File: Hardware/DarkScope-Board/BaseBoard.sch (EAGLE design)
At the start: 87 parts, among them IC1 7805DT, IC2 REG1117, IC3 7905, J1 DCJ0202, Q1 8MHz, T2 9014, U1 STM32F103CBT6, X1 TSW-102-07-G-S, X2 TSW-102-07-G-S, X3 MINI-USB-32005-301, X4 2540-5

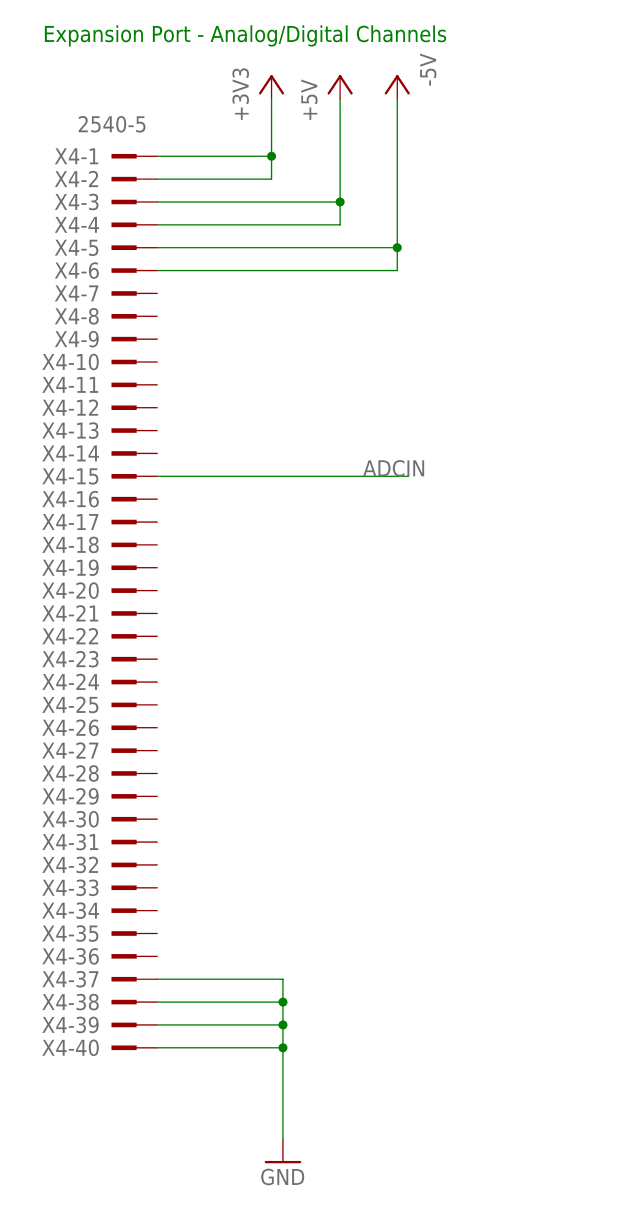
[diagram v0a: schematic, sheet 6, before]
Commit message: BaseBoard Schematic Complete
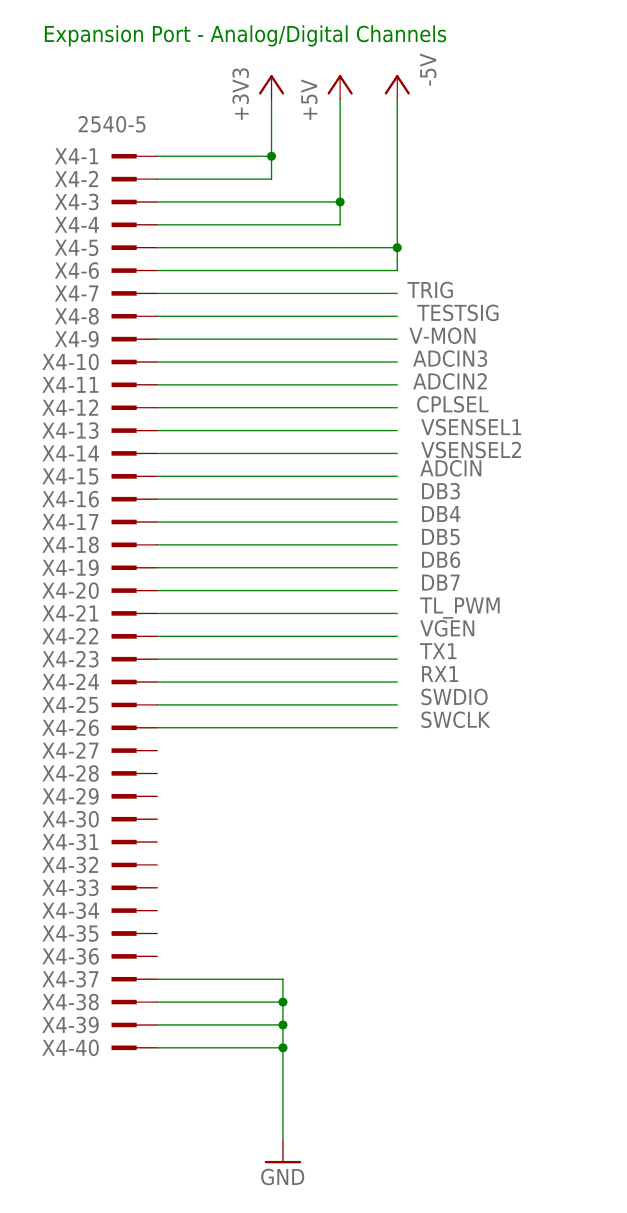
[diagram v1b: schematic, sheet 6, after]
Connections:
- net ADCIN2: now also X4-11.KL
- net ADCIN3: now also X4-10.KL
- net CPLSEL: now also X4-12.KL
- net DB3: now also X4-16.KL
- net DB4: now also X4-17.KL
- net DB5: now also X4-18.KL
- net DB6: now also X4-19.KL
- net DB7: now also X4-20.KL
- net RX1: now also X4-24.KL
- net SWCLK: now also X4-26.KL
- net SWDIO: now also X4-25.KL
- net TESTSIG: now also X4-8.KL
- net TL_PWM: now also X4-21.KL
- net TRIG: now also X4-7.KL
- net TX1: now also X4-23.KL
- net V-MON: now also X4-9.KL
- net VGEN: now also X4-22.KL
- net VSENSEL1: now also X4-13.KL
- net VSENSEL2: now also X4-14.KL
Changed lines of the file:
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@@
 <segment>
 <pinref part="X4" gate="-15" pin="KL"/>
-<wire x1="38.1" y1="53.34" x2="66.04" y2="53.34" width="0.1524" layer="91"/>
-<label x="60.96" y="53.34" size="1.778" layer="95"/>
+<wire x1="38.1" y1="53.34" x2="64.77" y2="53.34" width="0.1524" layer="91"/>
+<label x="67.31" y="53.34" size="1.778" layer="95"/>
 </segment>
 </net>
+<net name="VSENSEL2" class="0">
+<segment>
+<wire x1="64.77" y1="55.88" x2="38.1" y2="55.88" width="0.1524" layer="91"/>
+<label x="78.74" y="57.15" size="1.778" layer="95" rot="R180"/>
+<pinref part="X4" gate="-14" pin="KL"/>
+</segment>
+</net>
+<net name="VSENSEL1" class="0">
+<segment>
+<wire x1="64.77" y1="58.42" x2="38.1" y2="58.42" width="0.1524" layer="91"/>
+<label x="78.74" y="59.69" size="1.778" layer="95" rot="R180"/>
+<pinref part="X4" gate="-13" pin="KL"/>
+</segment>
+</net>
+<net name="CPLSEL" class="0">
+<segment>
+<wire x1="64.77" y1="60.96" x2="38.1" y2="60.96" width="0.1524" layer="91"/>
+<label x="74.93" y="62.23" size="1.778" layer="95" rot="R180"/>
+<pinref part="X4" gate="-12" pin="KL"/>
+</segment>
+</net>
+<net name="ADCIN2" class="0">
+<segment>
+<wire x1="64.77" y1="63.5" x2="38.1" y2="63.5" width="0.1524" layer="91"/>
+<label x="74.93" y="64.77" size="1.778" layer="95" rot="R180"/>
+<pinref part="X4" gate="-11" pin="KL"/>
+</segment>
+</net>
+<net name="ADCIN3" class="0">
+<segment>
+<wire x1="64.77" y1="66.04" x2="38.1" y2="66.04" width="0.1524" layer="91"/>
+<label x="74.93" y="67.31" size="1.778" layer="95" rot="R180"/>
+<pinref part="X4" gate="-10" pin="KL"/>
+</segment>
+</net>
+<net name="V-MON" class="0">
+<segment>
+<wire x1="64.77" y1="68.58" x2="38.1" y2="68.58" width="0.1524" layer="91"/>
+<label x="73.66" y="69.85" size="1.778" layer="95" rot="R180"/>
+<pinref part="X4" gate="-9" pin="KL"/>
+</segment>
+</net>
+<net name="TESTSIG" class="0">
+<segment>
+<wire x1="64.77" y1="71.12" x2="38.1" y2="71.12" width="0.1524" layer="91"/>
+<label x="76.2" y="72.39" size="1.778" layer="95" rot="R180"/>
+<pinref part="X4" gate="-8" pin="KL"/>
+</segment>
+</net>
+<net name="TRIG" class="0">
+<segment>
+<wire x1="64.77" y1="73.66" x2="38.1" y2="73.66" width="0.1524" layer="91"/>
+<label x="71.12" y="74.93" size="1.778" layer="95" rot="R180"/>
+<pinref part="X4" gate="-7" pin="KL"/>
+</segment>
+</net>
+<net name="DB3" class="0">
+<segment>
+<wire x1="38.1" y1="50.8" x2="64.77" y2="50.8" width="0.1524" layer="91"/>
+<label x="67.31" y="50.8" size="1.778" layer="95"/>
+<pinref part="X4" gate="-16" pin="KL"/>
+</segment>
+</net>
+<net name="DB4" class="0">
+<segment>
+<wire x1="38.1" y1="48.26" x2="64.77" y2="48.26" width="0.1524" layer="91"/>
+<label x="67.31" y="48.26" size="1.778" layer="95"/>
+<pinref part="X4" gate="-17" pin="KL"/>
+</segment>
+</net>
+<net name="DB5" class="0">
+<segment>
+<wire x1="38.1" y1="45.72" x2="64.77" y2="45.72" width="0.1524" layer="91"/>
+<label x="67.31" y="45.72" size="1.778" layer="95"/>
+<pinref part="X4" gate="-18" pin="KL"/>
+</segment>
+</net>
+<net name="DB6" class="0">
+<segment>
+<wire x1="38.1" y1="43.18" x2="64.77" y2="43.18" width="0.1524" layer="91"/>
+<label x="67.31" y="43.18" size="1.778" layer="95"/>
+<pinref part="X4" gate="-19" pin="KL"/>
+</segment>
+</net>
+<net name="DB7" class="0">
+<segment>
+<wire x1="38.1" y1="40.64" x2="64.77" y2="40.64" width="0.1524" layer="91"/>
+<label x="67.31" y="40.64" size="1.778" layer="95"/>
+<pinref part="X4" gate="-20" pin="KL"/>
+</segment>
+</net>
+<net name="TL_PWM" class="0">
+<segment>
+<wire x1="38.1" y1="38.1" x2="64.77" y2="38.1" width="0.1524" layer="91"/>
+<label x="67.31" y="38.1" size="1.778" layer="95"/>
+<pinref part="X4" gate="-21" pin="KL"/>
+</segment>
+</net>
+<net name="VGEN" class="0">
+<segment>
+<wire x1="38.1" y1="35.56" x2="64.77" y2="35.56" width="0.1524" layer="91"/>
+<label x="67.31" y="35.56" size="1.778" layer="95"/>
+<pinref part="X4" gate="-22" pin="KL"/>
+</segment>
+</net>
+<net name="TX1" class="0">
+<segment>
+<pinref part="X4" gate="-23" pin="KL"/>
+<wire x1="38.1" y1="33.02" x2="64.77" y2="33.02" width="0.1524" layer="91"/>
+<label x="67.31" y="33.02" size="1.778" layer="95"/>
+</segment>
+</net>
+<net name="RX1" class="0">
+<segment>
+<pinref part="X4" gate="-24" pin="KL"/>
+<wire x1="38.1" y1="30.48" x2="64.77" y2="30.48" width="0.1524" layer="91"/>
+<label x="67.31" y="30.48" size="1.778" layer="95"/>
+</segment>
+</net>
+<net name="SWDIO" class="0">
+<segment>
+<pinref part="X4" gate="-25" pin="KL"/>
+<wire x1="38.1" y1="27.94" x2="64.77" y2="27.94" width="0.1524" layer="91"/>
+<label x="67.31" y="27.94" size="1.778" layer="95"/>
+</segment>
+</net>
+<net name="SWCLK" class="0">
+<segment>
+<pinref part="X4" gate="-26" pin="KL"/>
+<wire x1="38.1" y1="25.4" x2="64.77" y2="25.4" width="0.1524" layer="91"/>
+<label x="67.31" y="25.4" size="1.778" layer="95"/>
+</segment>
+</net>

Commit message: DP
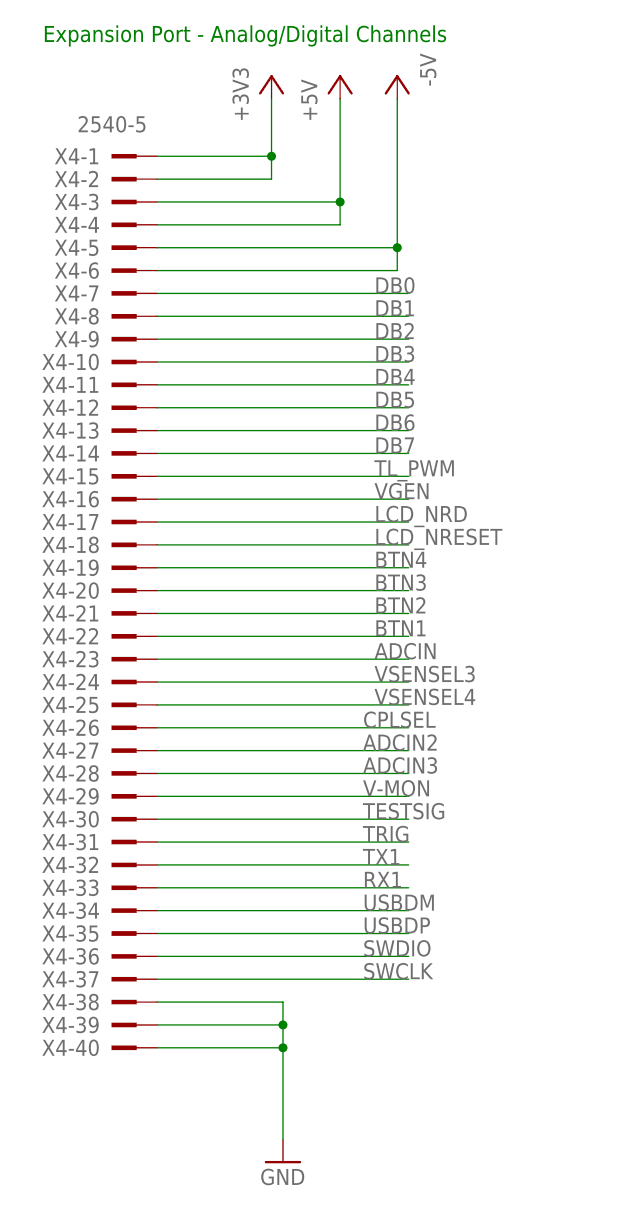
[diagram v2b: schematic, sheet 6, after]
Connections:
- new net VSENSEL3: X4-24.KL
- new net VSENSEL4: X4-25.KL
- net ADCIN: now also X4-23.KL; no longer X4-15.KL
- net ADCIN2: now also X4-27.KL; no longer X4-11.KL
- net ADCIN3: now also X4-28.KL; no longer X4-10.KL
- net BTN1: now also X4-22.KL
- net BTN2: now also X4-21.KL
- net BTN3: now also X4-20.KL
- net BTN4: now also X4-19.KL
- net CPLSEL: now also X4-26.KL; no longer X4-12.KL
- net DB0: now also X4-7.KL
- net DB1: now also X4-8.KL
- net DB2: now also X4-9.KL
- net DB3: now also X4-10.KL; no longer X4-16.KL
- net DB4: now also X4-11.KL; no longer X4-17.KL
- net DB5: now also X4-12.KL; no longer X4-18.KL
- net DB6: now also X4-13.KL; no longer X4-19.KL
- net DB7: now also X4-14.KL; no longer X4-20.KL
- net GND: no longer X4-37.KL
- net LCD_NRD: now also X4-17.KL
- net LCD_NRESET: now also X4-18.KL
- net RX1: now also X4-33.KL; no longer X4-24.KL
- net SWCLK: now also X4-37.KL; no longer X4-26.KL
- net SWDIO: now also X4-36.KL; no longer X4-25.KL
- net TESTSIG: now also X4-30.KL; no longer X4-8.KL
- net TL_PWM: now also X4-15.KL; no longer X4-21.KL
- net TRIG: now also X4-31.KL; no longer X4-7.KL
- net TX1: now also X4-32.KL; no longer X4-23.KL
- net USBDM: now also X4-34.KL
- net USBDP: now also X4-35.KL
- net V-MON: now also X4-29.KL; no longer X4-9.KL
- net VGEN: now also X4-16.KL; no longer X4-22.KL
- net VSENSEL1: no longer X4-13.KL
- net VSENSEL2: no longer X4-14.KL
